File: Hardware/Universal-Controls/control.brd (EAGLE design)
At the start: 32.7 x 46.2 mm, 44 parts, among them U1 STM32-M-64-LQFP, U2 MIC5233-5.0YM5-TR, U3 MIC5233-3.3YM5-TR, U4 TJA1042HVSON, U6 MCP6002, Y1 16MHz

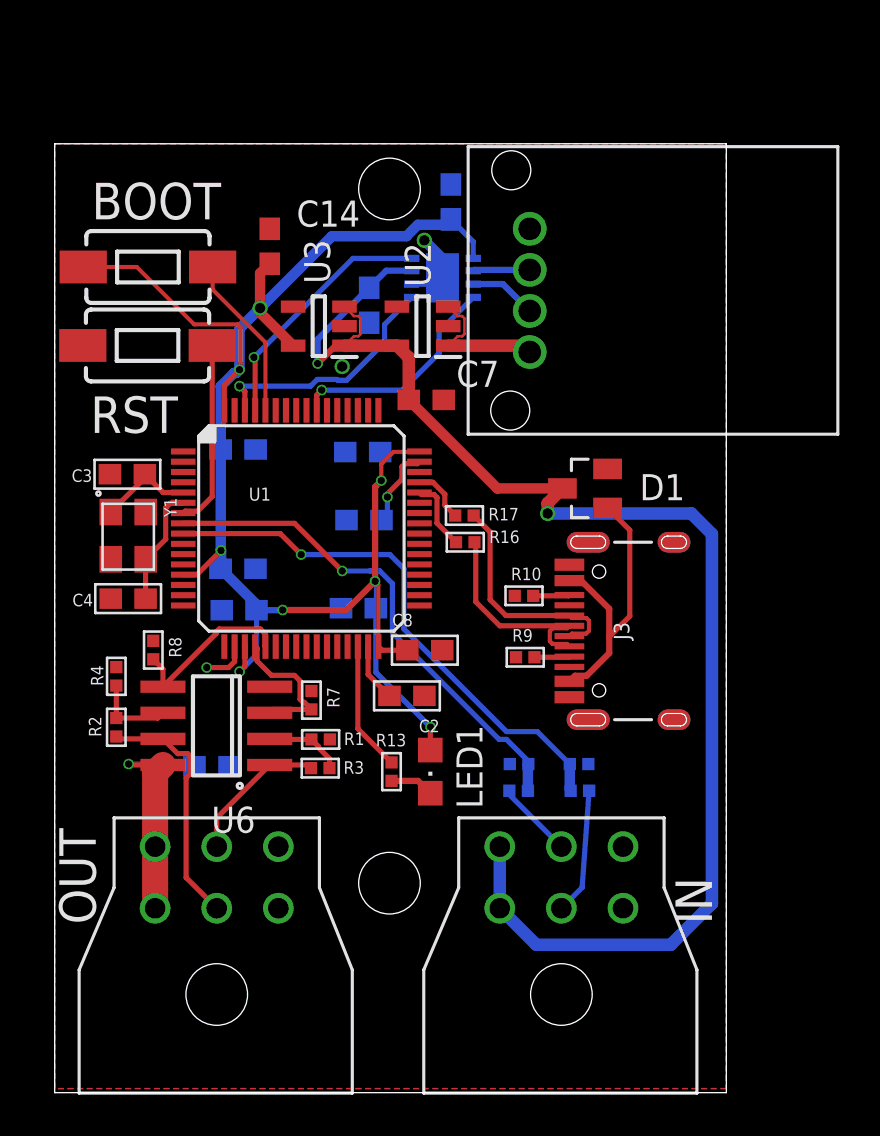
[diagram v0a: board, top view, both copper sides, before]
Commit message: Button controller commit
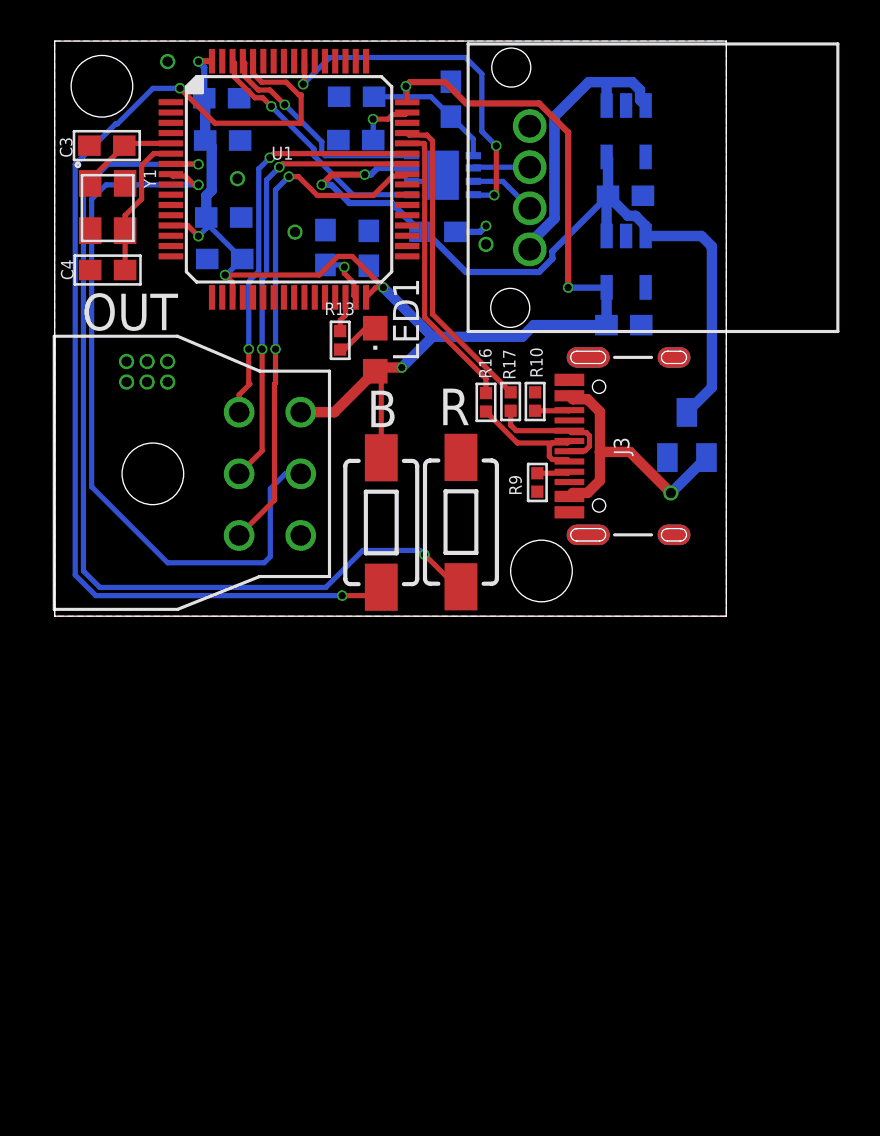
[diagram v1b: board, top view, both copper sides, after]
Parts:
- removed C26: 100nF, comma.ai:0603-C
- removed R1, R2, R3, R4, R7, R8: 10k, comma.ai:0402-R
- removed R23, R24, R25, R26: 1k, comma.ai:0402-R
- removed U$1: MICROFIT-6, interceptor:MICROFIT-6
- removed U6: MCP6002, comma.ai:SO08
- moved C8 26.7 mm to (8.18, 46.2), flipped to the bottom, turned to 180 degrees
- moved C2 22.2 mm to (13.2, 41.0), flipped to the bottom, turned to 270 degrees
- moved U$3 22.1 mm to (12.0, 29.9), turned to 270 degrees
- moved R13 21.1 mm to (13.9, 36.4)
- moved LED1 20.7 mm to (15.6, 36.0), turned to 0 degrees
- moved C1 18.5 mm to (14.7, 46.2)
- moved C14 17.7 mm to (27.7, 37.2), flipped to the bottom, turned to 180 degrees
- moved C11 17.5 mm to (15.3, 40.9), turned to 90 degrees
- moved S1 17.5 mm to (19.8, 27.6), turned to 270 degrees
- moved C10 17.3 mm to (14.7, 48.3)
- moved C9 17.1 mm to (8.13, 48.2)
- moved C12 17.1 mm to (8.28, 40.4)
- moved C13 17.1 mm to (8.23, 42.4)
- moved U1 17.0 mm to (11.4, 44.3)
- moved S2 16.8 mm to (15.9, 27.6), turned to 270 degrees
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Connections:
- removed net ACCEL1: R23.2, U$3.2
- removed net ACCEL2: R24.2, U$3.5
- removed net DAC1: R3.2, U$1.2, U6.1
- removed net DAC2: R2.2, U$1.5, U6.7
- removed net DACV: C26.1, U$1.3, U$1.6, U6.8
- removed net N$17: R7.2, U1.20, U6.3
- removed net N$18: R8.2, U1.21, U6.5
- removed net N$21: R1.2, R3.1, U6.2
- removed net N$22: R2.1, R4.2, U6.6
- removed net N$41: R23.1, R26.1, U1.8
- removed net N$42: R24.1, R25.1, U1.9
- new net ADC: U$3.2, U1.8
- new net ENC1: U$3.4, U1.41
- new net ENC2: U$3.5, U1.42
- new net IO1: U$3.6, U1.43
- net 3V3: now also U$3.3
- net 5V: no longer U$3.3, U$3.6
- net GND: no longer C26.2, R1.1, R25.2, R26.2, R4.1, R7.1, R8.1, U$1.1, U$1.4, U$3.4, U6.4
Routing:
- net N$7: track 8.04 -> 53.5 mm, vias 0 -> 2
- net N$10: track 9.10 -> 46.2 mm, vias 0 -> 2
- net ADC: track 0.00 -> 36.5 mm, vias 0 -> 1
- net 5V: track 69.1 -> 41.0 mm
- net N$42: track 26.5 -> 0.00 mm, vias 1 -> 0
- net ENC1: track 0.00 -> 25.0 mm, vias 0 -> 2
- net N$41: track 24.5 -> 0.00 mm, vias 1 -> 0
- net ENC2: track 0.00 -> 22.0 mm, vias 0 -> 2
- net IO1: track 0.00 -> 19.8 mm, vias 0 -> 2
- net N$4: track 2.72 -> 15.2 mm
- net DAC2: track 12.1 -> 0.00 mm
- net DACV: track 12.1 -> 0.00 mm, vias 1 -> 0
- net N$2: track 3.51 -> 14.2 mm
- net N$18: track 8.44 -> 0.00 mm
- net 12V: track 6.91 -> 14.1 mm
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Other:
- board size 32.7 x 46.2 mm -> 32.7 x 28 mm
- board text added: "B"
- board text added: "R"
- board text removed: "BOOT"
- board text removed: "IN"
- board text removed: "RST"
